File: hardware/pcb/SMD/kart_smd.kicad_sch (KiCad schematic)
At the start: 20 parts, among them J1 GPS, J2 I2S AMP, J3 Battery, Q1 BC327, Q2 2N3904, Q4 2N3904, SW1 ON/OFF, U2 XIAO-ESP32-S3-SMD

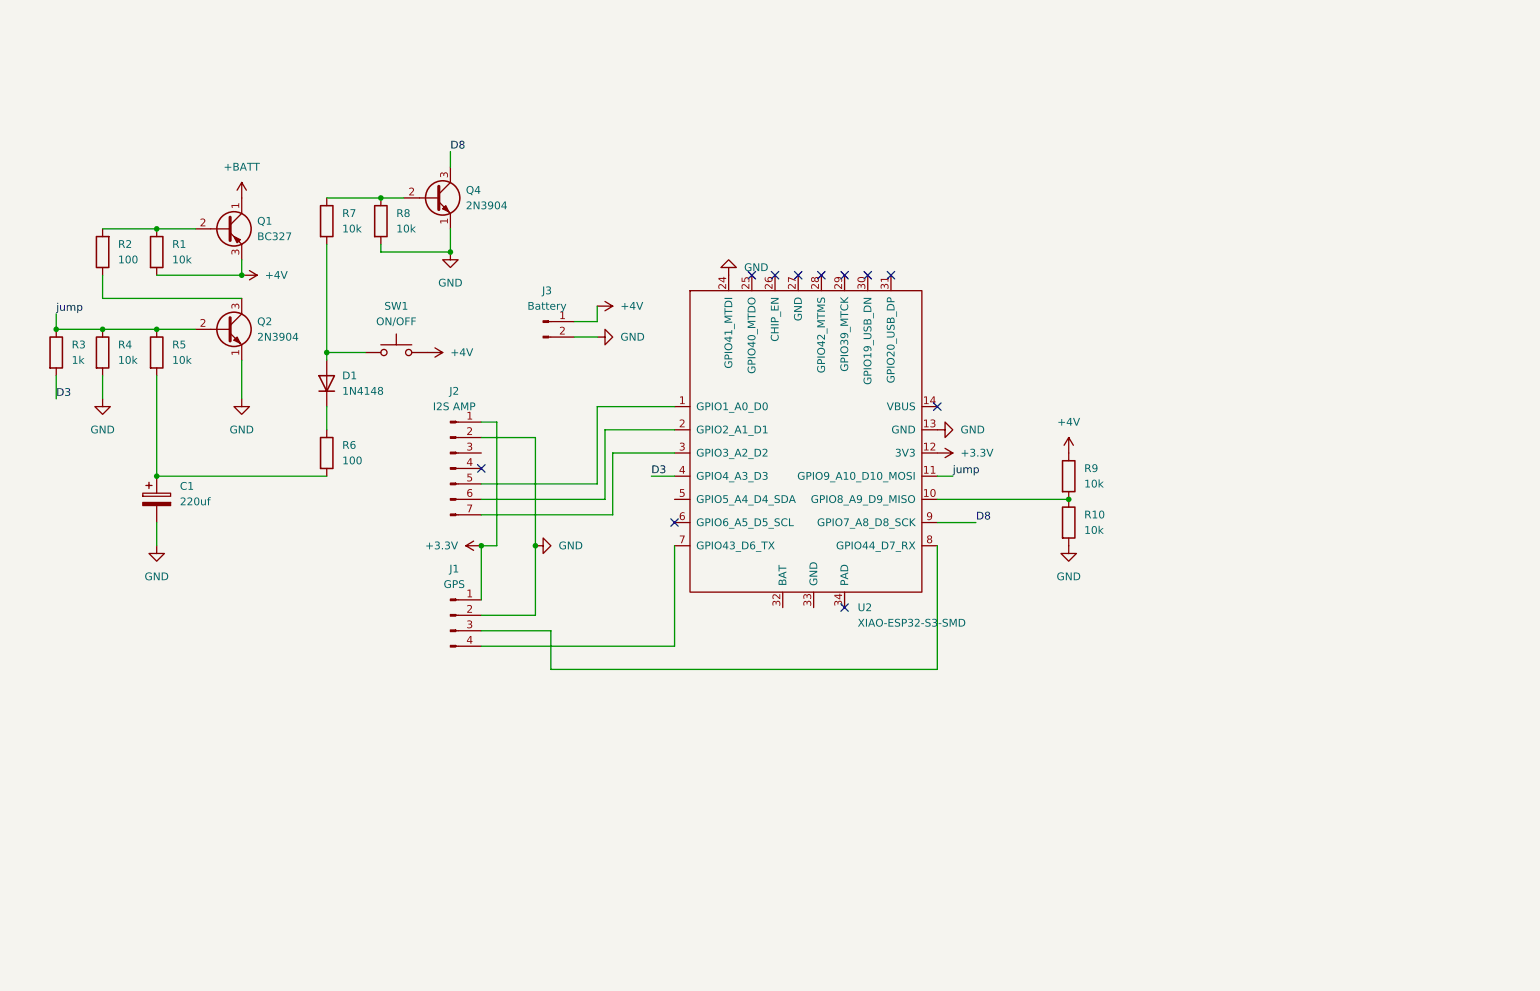
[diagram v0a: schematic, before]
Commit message: software version 1 used on a real kart on 2026/03/26
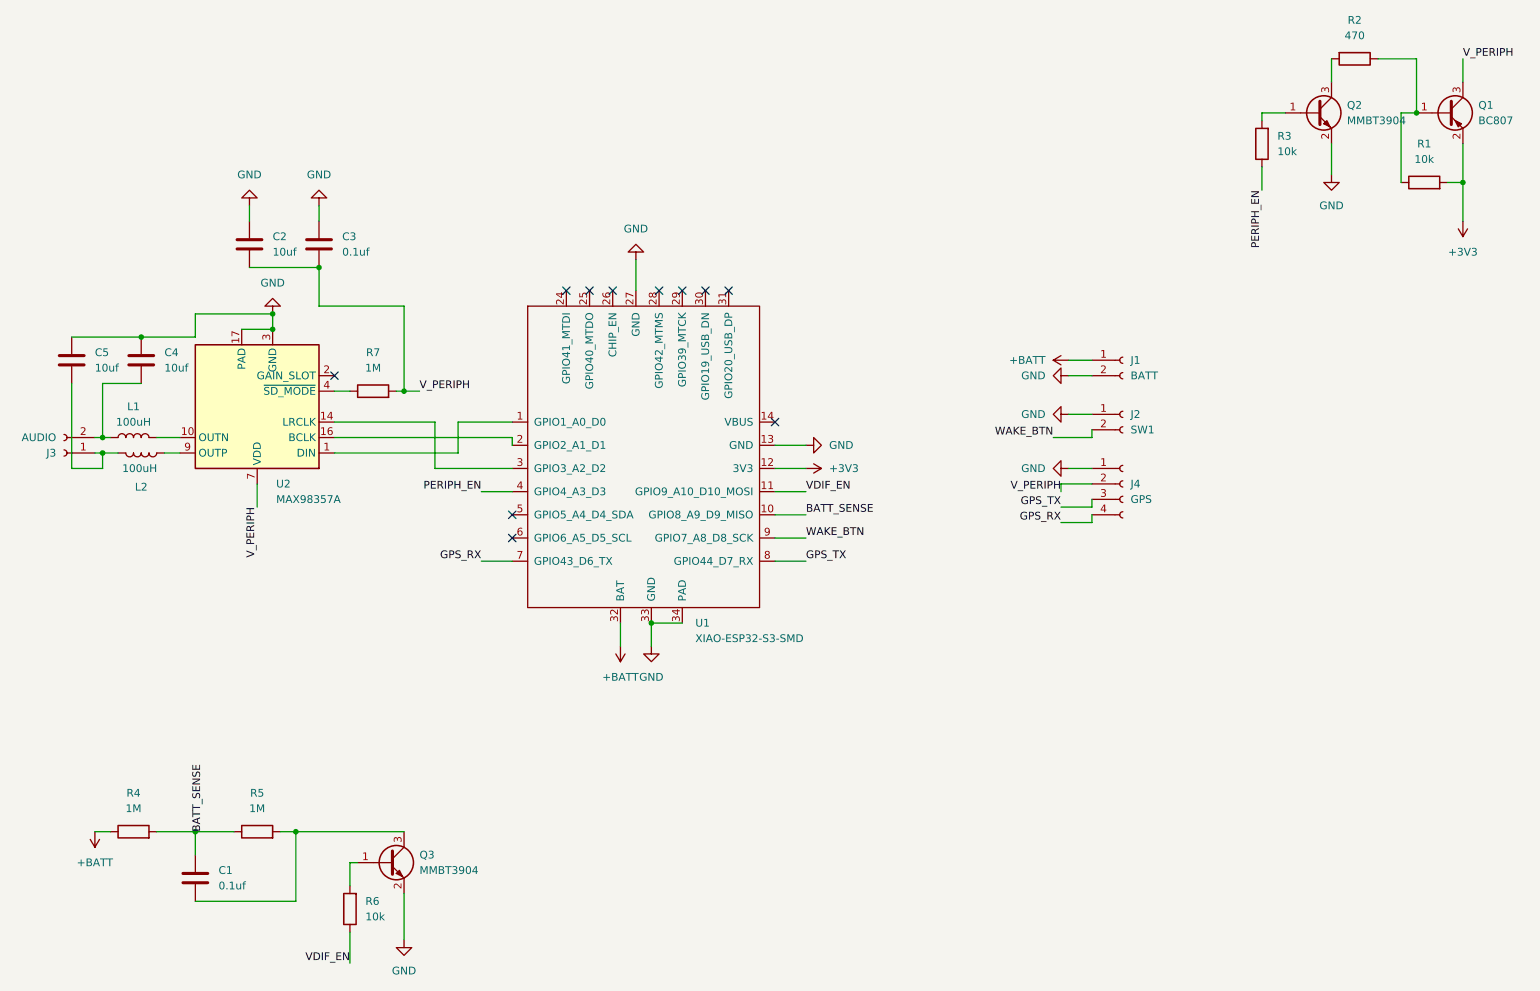
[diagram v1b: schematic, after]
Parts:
- removed C1: 220uf, Capacitor_THT:CP_Radial_D6.3mm_P2.50mm, symbol Device:C_Polarized
- removed D1: 1N4148, Diode_THT:D_DO-34_SOD68_P7.62mm_Horizontal, symbol Diode:1N4148
- removed J1: GPS, Connector_PinHeader_2.54mm:PinHeader_1x04_P2.54mm_Vertical, symbol Connector:Conn_01x04_Pin
- removed J2: I2S AMP, Connector_PinHeader_2.54mm:PinHeader_1x07_P2.54mm_Vertical, symbol Connector:Conn_01x07_Pin
- removed J3: Battery, Connector_PinHeader_2.54mm:PinHeader_1x02_P2.54mm_Vertical, symbol Connector:Conn_01x02_Pin
- removed Q1: BC327, Package_TO_SOT_THT:TO-92_Inline_Wide, symbol Transistor_BJT:BC327
- removed Q2, Q4: 2N3904, Package_TO_SOT_THT:TO-92_Inline_Wide, symbol Transistor_BJT:2N3904
- removed R10, R8, R9: 10k, Resistor_THT:R_Axial_DIN0207_L6.3mm_D2.5mm_P7.62mm_Horizontal, symbol Device:R
- removed SW1: ON/OFF, Connector_PinHeader_2.54mm:PinHeader_1x02_P2.54mm_Vertical, symbol Switch:SW_Push
- removed U2: XIAO-ESP32-S3-SMD, Seeed Fusion Component Libraries for KiCad:XIAO-ESP32-S3-SMD, symbol Seeed_Studio_XIAO_Series:XIAO-ESP32-S3-SMD
- added C1, C3: 0.1uf, Capacitor_SMD:C_0805_2012Metric, symbol Device:C
- added C2, C4, C5: 10uf, Capacitor_SMD:C_0805_2012Metric, symbol Device:C
- added J1: BATT, Connector_JST:JST_PH_S2B-PH-K_1x02_P2.00mm_Horizontal, symbol Connector:Conn_01x02_Socket
- added J2: SW1, Connector_JST:JST_PH_S2B-PH-K_1x02_P2.00mm_Horizontal, symbol Connector:Conn_01x02_Socket
- added J3: AUDIO, Connector_JST:JST_PH_S2B-PH-K_1x02_P2.00mm_Horizontal, symbol Connector:Conn_01x02_Socket
- added J4: GPS, Connector_JST:JST_PH_S4B-PH-K_1x04_P2.00mm_Horizontal, symbol Connector:Conn_01x04_Socket
- added L1, L2: 100uH, Inductor_SMD:L_0805_2012Metric, symbol Device:L
- added Q1: BC807, Package_TO_SOT_SMD:SOT-23, symbol Transistor_BJT:BC807
- added Q2, Q3: MMBT3904, Package_TO_SOT_SMD:SOT-23, symbol Transistor_BJT:MMBT3904
- added U1: XIAO-ESP32-S3-SMD, Seeed_Studio_XIAO_Series:XIAO-ESP32-S3-SMD, symbol Seeed_Studio_XIAO_Series:XIAO-ESP32-S3-SMD
- added U2: MAX98357A, Package_DFN_QFN:TQFN-16-1EP_3x3mm_P0.5mm_EP1.23x1.23mm_ThermalVias, symbol Audio:MAX98357A
- R1: footprint Resistor_THT:R_Axial_DIN0207_L6.3mm_D2.5mm_P7.62mm_Horizontal -> Resistor_SMD:R_0805_2012Metric
- R2: value 100 -> 470; footprint Resistor_THT:R_Axial_DIN0207_L6.3mm_D2.5mm_P7.62mm_Horizontal -> Resistor_SMD:R_0805_2012Metric
- R3: value 1k -> 10k; footprint Resistor_THT:R_Axial_DIN0207_L6.3mm_D2.5mm_P7.62mm_Horizontal -> Resistor_SMD:R_0805_2012Metric
- R4, R5, R7: value 10k -> 1M; footprint Resistor_THT:R_Axial_DIN0207_L6.3mm_D2.5mm_P7.62mm_Horizontal -> Resistor_SMD:R_0805_2012Metric
- R6: value 100 -> 10k; footprint Resistor_THT:R_Axial_DIN0207_L6.3mm_D2.5mm_P7.62mm_Horizontal -> Resistor_SMD:R_0805_2012Metric
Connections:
- net +BATT: now also R4.1, J1.1 (Pin_1), U1.32 (BAT)
- net GND: now also C2.1, C3.1, C4.1, C5.1, J1.2 (Pin_2), J2.1 (Pin_1), J4.1 (Pin_1), Q2.2 (E), Q3.2 (E), U1.13 (GND), U1.27 (GND), U1.33 (GND), U1.34 (PAD), U2.11 (GND), U2.15 (GND), U2.17 (PAD), U2.3 (GND); no longer R4.2
- net VDIF_EN: now reaches R6.1
- net VDIF_EN: now also U1.11 (GPIO9_A10_D10_MOSI)
- net at R6.2: now also Q3.1 (B); no longer R5.2
- net V_PERIPH: now reaches R7.2
- net V_PERIPH: now also C2.2, C3.2, J4.2 (Pin_2), Q1.3 (C), U2.7 (VDD), U2.8 (VDD)
- net at R2.1: now also R1.1, Q1.1 (B)
- net at R2.2: now also Q2.3 (C); no longer R1.1
- net at R7.1: now also U2.4 (~{SD_MODE})
- net +4V renamed +3V3
- net +3V3: now also Q1.2 (E), U1.12 (3V3)
- net D3: no longer names the net of R3.2
- net D3: now also Q2.1 (B)
- removed net jump: R3.1, R4.1, R5.1
- new net: C1.1, Q3.3 (C), R5.2
- new net: C4.2, J3.2 (Pin_2), L1.1
- new net: L2.1, U2.9 (OUTP)
- new net: C5.2, J3.1 (Pin_1), L2.2
- new net: U1.1 (GPIO1_A0_D0), U2.1 (DIN)
- new net: U1.2 (GPIO2_A1_D1), U2.16 (BCLK)
- new net: U1.3 (GPIO3_A2_D2), U2.14 (LRCLK)
- new net: L1.2, U2.10 (OUTN)
- new net BATT_SENSE: C1.2, R4.2, R5.1, U1.10 (GPIO8_A9_D9_MISO)
- new net GPS_RX: J4.4 (Pin_4), U1.7 (GPIO43_D6_TX)
- new net GPS_TX: J4.3 (Pin_3), U1.8 (GPIO44_D7_RX)
- new net PERIPH_EN: R3.1, U1.4 (GPIO4_A3_D3)
- new net WAKE_BTN: J2.2 (Pin_2), U1.9 (GPIO7_A8_D8_SCK)
